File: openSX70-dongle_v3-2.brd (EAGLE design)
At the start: 47.1 x 24.7 mm, 24 parts

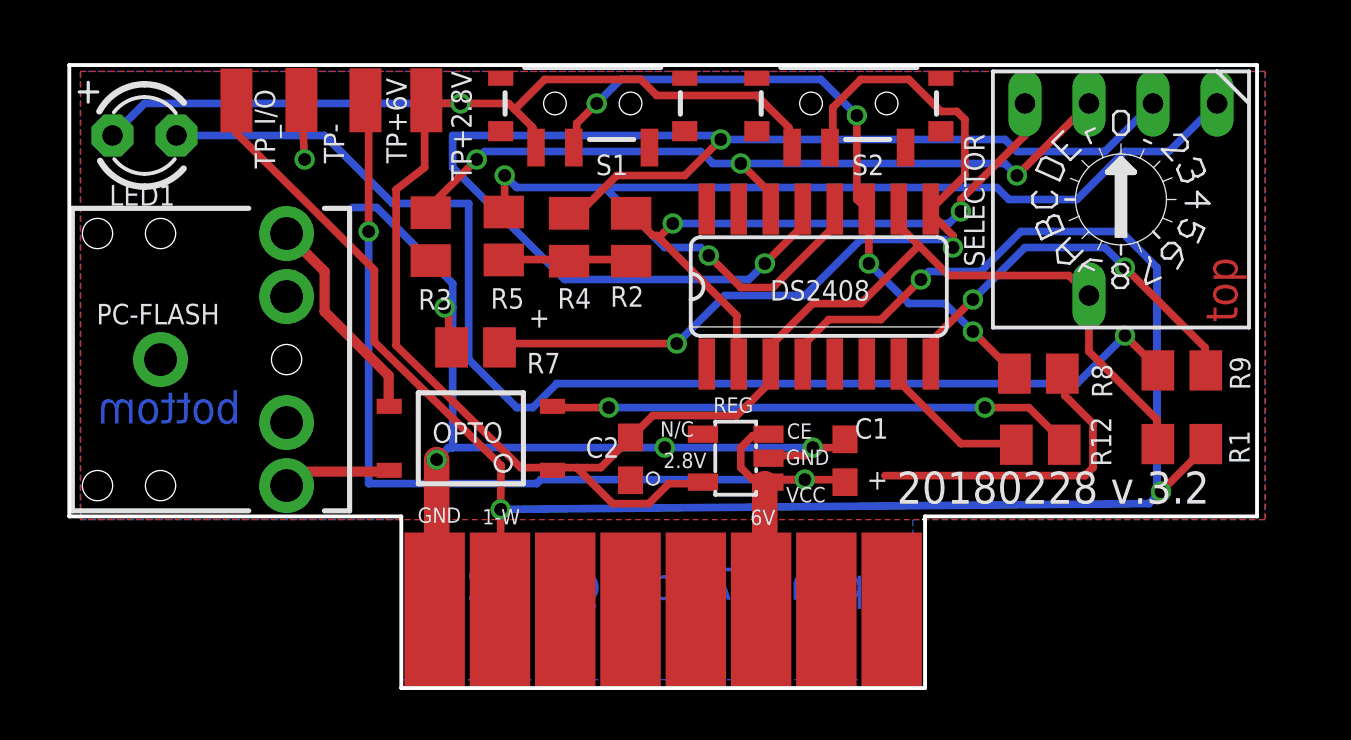
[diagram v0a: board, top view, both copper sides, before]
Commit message: New Gerbers, ready to order!
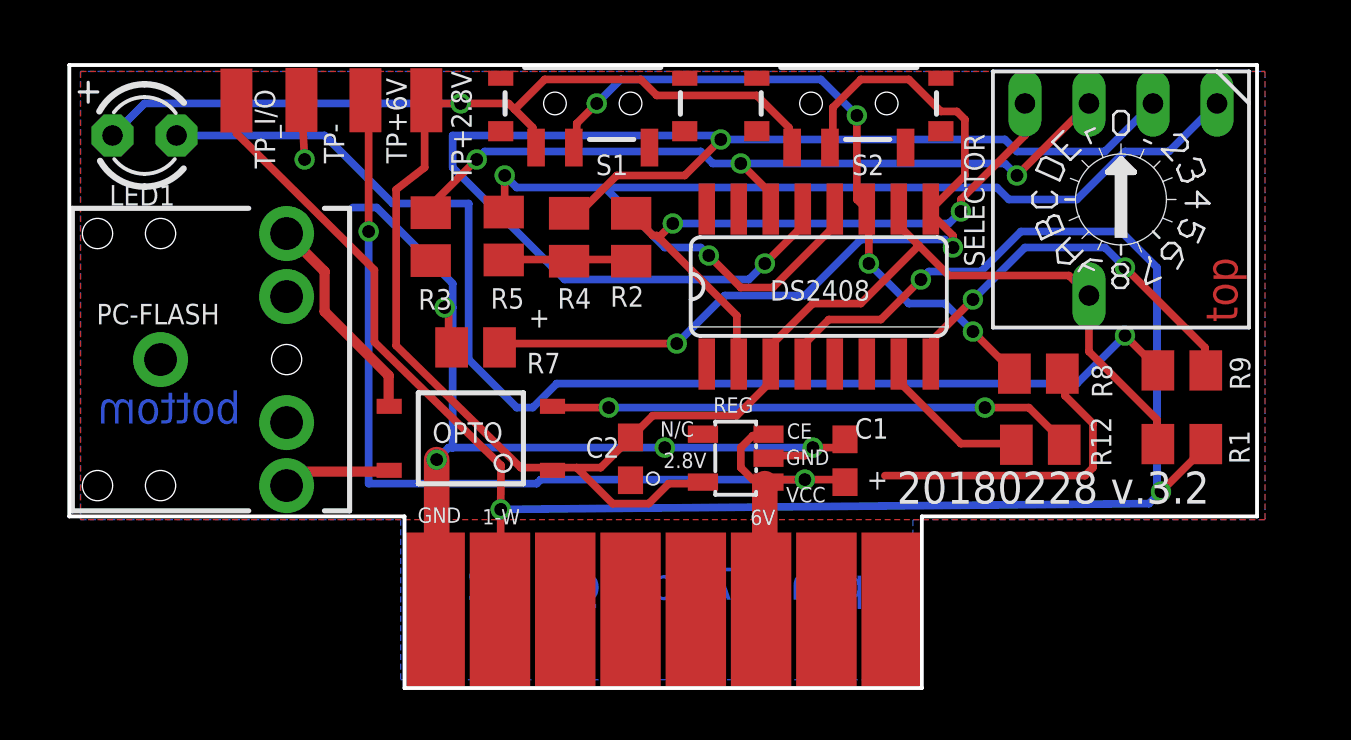
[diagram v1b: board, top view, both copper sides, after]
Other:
- outline, holes or cut-outs redrawn
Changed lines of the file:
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@@
 <layer number="20" name="Dimension" color="24" fill="1" visible="yes" active="yes"/>
 <layer number="21" name="tPlace" color="7" fill="1" visible="yes" active="yes"/>
-<layer number="22" name="bPlace" color="7" fill="1" visible="no" active="yes"/>
+<layer number="22" name="bPlace" color="7" fill="1" visible="yes" active="yes"/>
 <layer number="23" name="tOrigins" color="15" fill="1" visible="yes" active="yes"/>
-<layer number="24" name="bOrigins" color="15" fill="1" visible="no" active="yes"/>
+<layer number="24" name="bOrigins" color="15" fill="1" visible="yes" active="yes"/>
 <layer number="25" name="tNames" color="7" fill="1" visible="yes" active="yes"/>
-<layer number="26" name="bNames" color="7" fill="1" visible="no" active="yes"/>
+<layer number="26" name="bNames" color="7" fill="1" visible="yes" active="yes"/>
 <layer number="27" name="tValues" color="7" fill="1" visible="no" active="yes"/>
 <layer number="28" name="bValues" color="7" fill="1" visible="no" active="yes"/>
@@
 <layer number="38" name="bTest" color="7" fill="1" visible="no" active="yes"/>
 <layer number="39" name="tKeepout" color="4" fill="11" visible="yes" active="yes"/>
-<layer number="40" name="bKeepout" color="1" fill="11" visible="no" active="yes"/>
+<layer number="40" name="bKeepout" color="1" fill="11" visible="yes" active="yes"/>
 <layer number="41" name="tRestrict" color="4" fill="10" visible="yes" active="yes"/>
-<layer number="42" name="bRestrict" color="1" fill="10" visible="no" active="yes"/>
+<layer number="42" name="bRestrict" color="1" fill="10" visible="yes" active="yes"/>
 <layer number="43" name="vRestrict" color="2" fill="10" visible="no" active="yes"/>
-<layer number="44" name="Drills" color="7" fill="1" visible="no" active="yes"/>
+<layer number="44" name="Drills" color="7" fill="1" visible="yes" active="yes"/>
 <layer number="45" name="Holes" color="7" fill="1" visible="yes" active="yes"/>
 <layer number="46" name="Milling" color="3" fill="1" visible="no" active="yes"/>
@@
 <layer number="50" name="dxf" color="7" fill="1" visible="no" active="no"/>
 <layer number="51" name="tDocu" color="7" fill="1" visible="yes" active="yes"/>
-<layer number="52" name="bDocu" color="7" fill="1" visible="no" active="yes"/>
+<layer number="52" name="bDocu" color="7" fill="1" visible="yes" active="yes"/>
 <layer number="53" name="tGND_GNDA" color="7" fill="9" visible="no" active="no"/>
 <layer number="54" name="bGND_GNDA" color="1" fill="9" visible="no" active="no"/>
@@
 <board>
 <plain>
-<wire x1="35.938" y1="7.62" x2="36.0426" y2="7.747" width="0.001" layer="20"/>
+<wire x1="35.938" y1="7.62" x2="35.9156" y2="7.747" width="0.001" layer="20"/>
 <text x="48.4378" y="15.4559" size="1.27" layer="1" font="vector" ratio="12" rot="R90">top</text>
 <text x="8.89" y="11.43" size="1.27" layer="16" font="vector" ratio="12" rot="MR0">bottom</text>
 <text x="34.6075" y="4.445" size="1.27" layer="16" font="vector" ratio="12" rot="MR0">openSX70 dongle 3.2</text>
 <text x="34.925" y="8.255" size="1.27" layer="21" font="vector">20180228 v.3.2</text>
-<wire x1="2.0955" y1="7.747" x2="15.2654" y2="7.747" width="0.1524" layer="20"/>
-<wire x1="15.2654" y1="7.747" x2="15.2654" y2="0.9398" width="0.1524" layer="20"/>
-<wire x1="15.2654" y1="0.9398" x2="36.0426" y2="0.9398" width="0.1524" layer="20"/>
-<wire x1="36.0426" y1="0.9398" x2="36.0426" y2="7.747" width="0.1524" layer="20"/>
-<wire x1="36.0426" y1="7.747" x2="49.2125" y2="7.747" width="0.1524" layer="20"/>
+<wire x1="2.0955" y1="7.747" x2="15.3924" y2="7.747" width="0.1524" layer="20"/>
+<wire x1="15.3924" y1="7.747" x2="15.3924" y2="0.9398" width="0.1524" layer="20"/>
+<wire x1="15.3924" y1="0.9398" x2="35.9156" y2="0.9398" width="0.1524" layer="20"/>
+<wire x1="35.9156" y1="0.9398" x2="35.9156" y2="7.747" width="0.1524" layer="20"/>
+<wire x1="35.9156" y1="7.747" x2="49.2125" y2="7.747" width="0.1524" layer="20"/>
 <wire x1="49.2125" y1="7.747" x2="49.2125" y2="25.654" width="0.1524" layer="20"/>
 <wire x1="49.2125" y1="25.654" x2="2.0955" y2="25.654" width="0.1524" layer="20"/>
@@
 <text x="20.32" y="15.24" size="0.8128" layer="21" font="vector" ratio="20">+</text>
 <text x="33.7312" y="8.8138" size="0.8128" layer="21" font="vector" ratio="20">+</text>
+<dimension x1="15.3924" y1="0.9398" x2="35.9156" y2="0.9398" x3="25.654" y3="-3.81" textsize="1.778" layer="1"/>
 </plain>
 <attributes>
